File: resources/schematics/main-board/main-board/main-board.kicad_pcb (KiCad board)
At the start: 2 copper layers, 53.3 x 30.5 mm, 6 parts, among them J1 Conn_01x02_Female, J2 Conn_01x04_Female, J3 Conn_01x03_Female

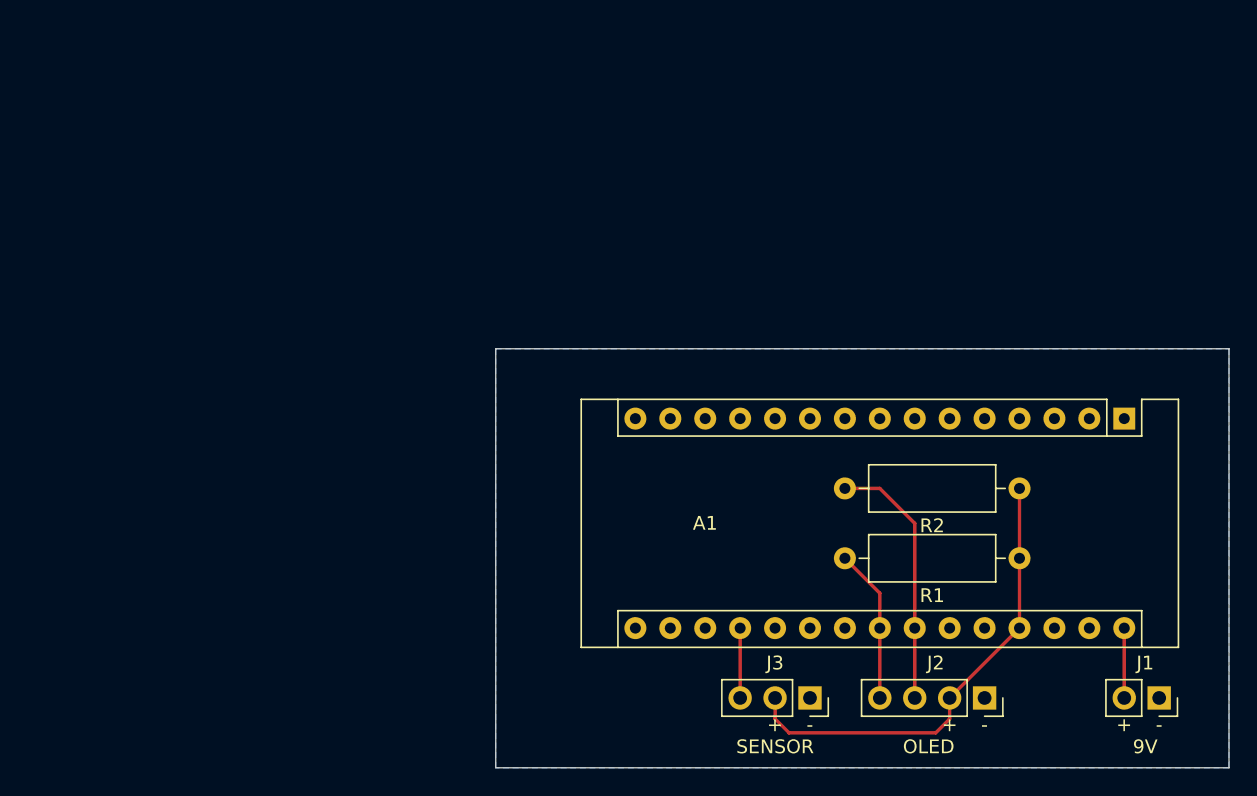
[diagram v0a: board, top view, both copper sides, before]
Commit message: Refactor PCB - batch-20201231
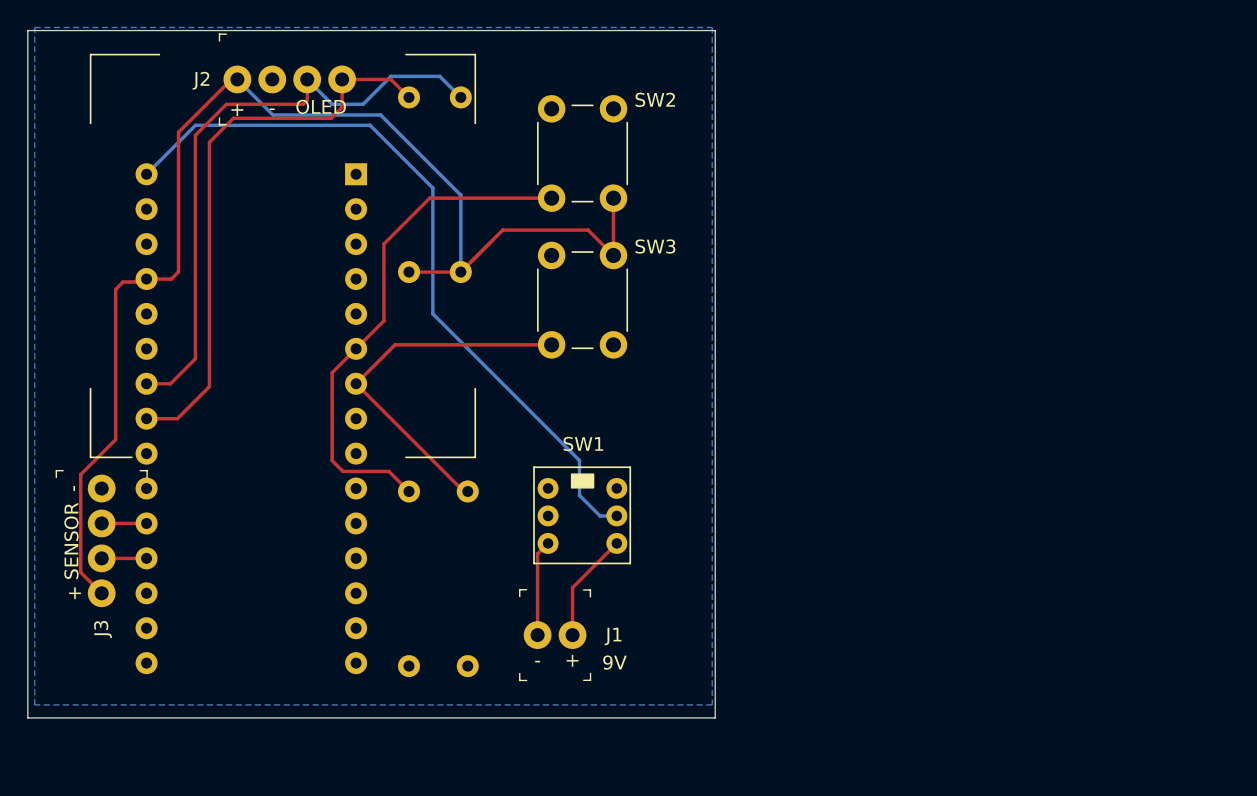
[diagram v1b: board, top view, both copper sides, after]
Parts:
- added R3: 10K, Resistor_THT:R_Axial_DIN0309_L9.0mm_D3.2mm_P12.70mm_Horizontal, B.Cu at (77.5, 96.7)
- added R4: 10K, Resistor_THT:R_Axial_DIN0309_L9.0mm_D3.2mm_P12.70mm_Horizontal, B.Cu at (81.8, 96.7)
- added SW1: SW_Push_DPDT, clvlabs:Switch_DPDT_7x7mm, F.Cu at (87.6, 83.8)
- added SW2: SW_Push_45deg, Button_Switch_THT:SW_PUSH_6mm_H7.3mm, F.Cu at (87.9, 62.7)
- added SW3: SW_Push_45deg, Button_Switch_THT:SW_PUSH_6mm_H7.3mm, F.Cu at (87.9, 73.4)
- A1, R1, R2: moved to B.Cu
- J1: footprint Connector_PinSocket_2.54mm:PinSocket_1x02_P2.54mm_Vertical -> digikey-footprints:PinHeader_1x2_P2.54mm_Drill1.02mm
- J2: footprint Connector_PinSocket_2.54mm:PinSocket_1x04_P2.54mm_Vertical -> digikey-footprints:PinHeader_1x4_P2.54mm_Drill1.02mm
- J3: value Conn_01x03_Female -> Conn_01x04_Female; footprint Connector_PinSocket_2.54mm:PinSocket_1x03_P2.54mm_Vertical -> digikey-footprints:PinHeader_1x4_P2.54mm_Drill1.02mm
- moved J2 70.6 mm to (65.0, 54.1), turned to 0 degrees
- moved A1 58.6 mm to (73.7, 61.0), turned to 180 degrees
- moved J3 53.7 mm to (55.2, 83.8)
- moved R1 49.0 mm to (77.5, 68.1), turned to 90 degrees
- moved J1 45.4 mm to (86.9, 94.5), turned to 0 degrees
- moved R2 43.6 mm to (81.3, 68.1), turned to 90 degrees
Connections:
- net DISTANCE_SENSOR_PIN renamed PING_TRIGGER_PIN
- A1 pad 20: Net-(A1-Pad20) -> PING_ECHO_PIN
- A1 pad 6: Net-(A1-Pad6) -> BUTTON_UP_PIN
- A1 pad 7: Net-(A1-Pad7) -> BUTTON_DOWN_PIN
- J1 pad 1: GND -> BATT_GND
- J1 pad 2: VIN -> BATT_VIN
- J2 pad 1: GND -> +5V
- J2 pad 2: +5V -> GND
- J3 pad 2: +5V -> PING_ECHO_PIN
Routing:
- net +5V: track 33.9 -> 94.6 mm
- net VIN: track 5.08 -> 54.3 mm
- net BUTTON_UP_PIN: track 0.00 -> 38.1 mm
- net I2C_SDA: track 11.2 -> 41.8 mm
- net BUTTON_DOWN_PIN: track 0.00 -> 27.5 mm
- net I2C_SCL: track 18.8 -> 45.2 mm
- net BATT_VIN: track 0.00 -> 8.00 mm
- net BATT_GND: track 0.00 -> 6.98 mm
- net PING_ECHO_PIN: track 0.00 -> 3.26 mm
- net PING_TRIGGER_PIN: track 5.08 -> 3.26 mm
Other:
- board size 53.3 x 30.5 mm -> 50 x 50 mm
- board text added: "20201231"
- board text added: "Arduino Nano"
- board text added: "github.com/clvLabs/gas-oil-tank-level"
